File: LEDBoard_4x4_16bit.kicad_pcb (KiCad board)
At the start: 2 copper layers, 40 x 40 mm, 35 parts, among them J1 signal_in, J2 power, J6 signal_out, U1 TLC5971RGER, U2 TLC5971RGER, U3 TLC5971RGER, U4 TLC5971RGER

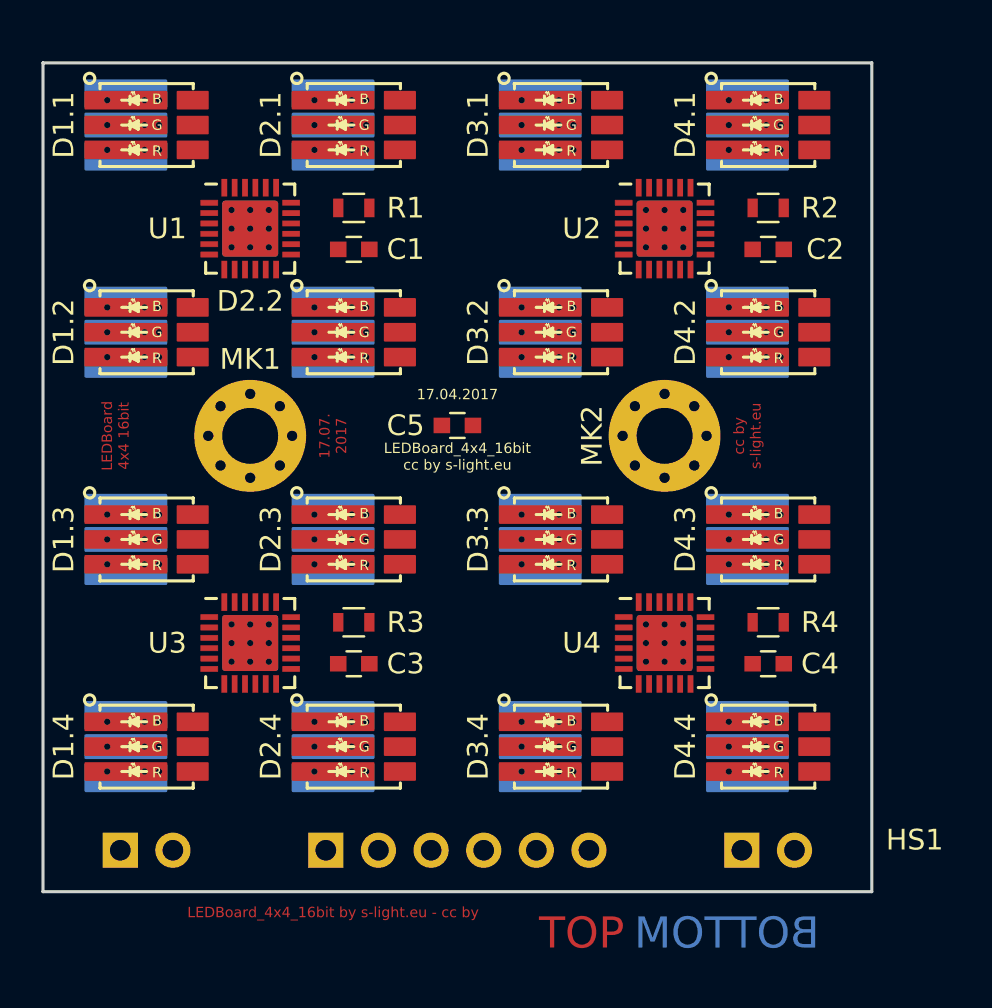
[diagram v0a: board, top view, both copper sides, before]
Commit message: pcb started routing
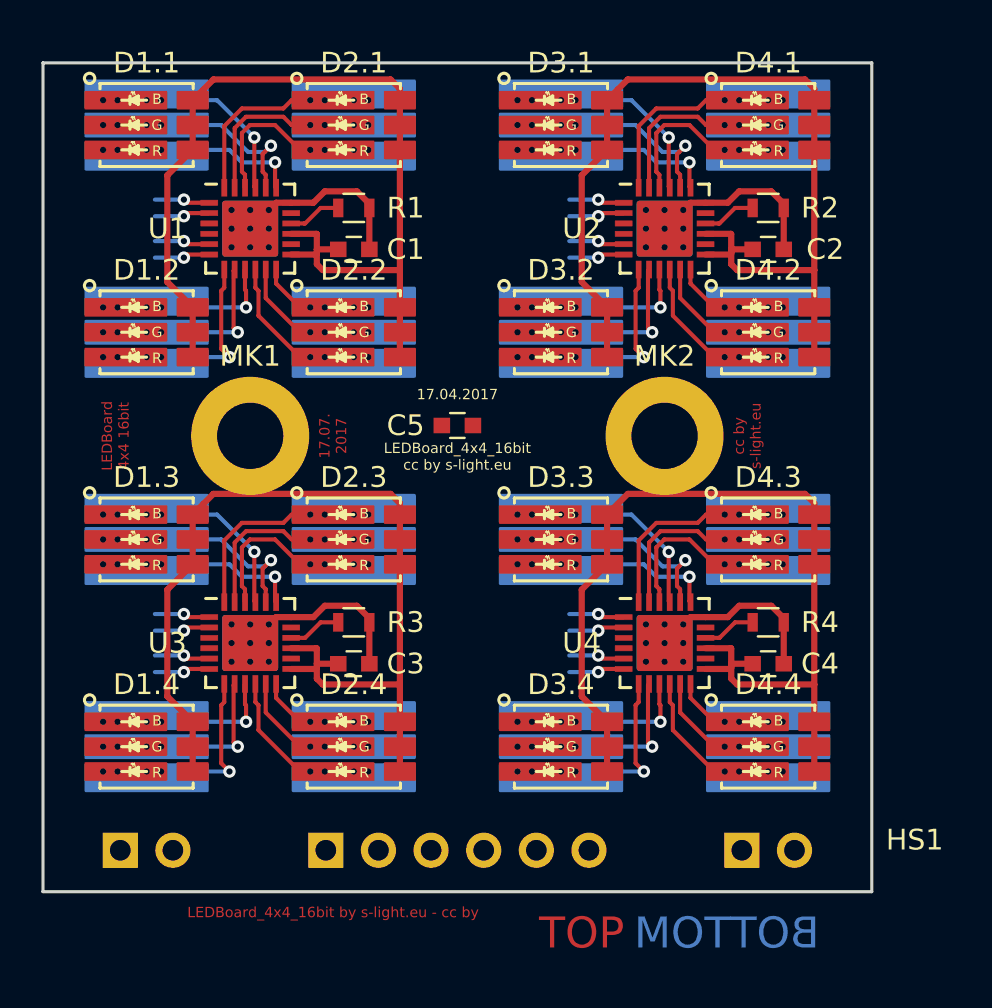
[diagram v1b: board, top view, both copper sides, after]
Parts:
- D1.1, D1.2, D1.3, D1.4, D2.1, D2.2, D2.3, D2.4, D3.1, D3.2, D3.3, D3.4, D4.1, D4.2, D4.3, D4.4: footprint nichia:LED_NSSM032AT_wViaHeatSink -> nichia:LED_NSSM032AT_wViaHeatSinkBig
- MK1, MK2: footprint Mounting_Holes:MountingHole_2.7mm_M2.5_Pad_Via -> Mounting_Holes:MountingHole_3.2mm_M3_ISO7380_Pad
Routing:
- net VCC: track 0.00 -> 184.3 mm
- net GND: track 0.00 -> 88.3 mm
- net /LED_3.1_G: track 0.00 -> 35.7 mm, vias 0 -> 4
- net /LED_4.1_B: track 0.00 -> 35.0 mm
- net /LED_3.2_R: track 0.00 -> 33.8 mm, vias 0 -> 4
- net /LED_3.1_B: track 0.00 -> 33.6 mm, vias 0 -> 4
- net /LED_4.1_G: track 0.00 -> 32.1 mm
- net /LED_4.1_R: track 0.00 -> 31.0 mm
- net /LED_3.1_R: track 0.00 -> 30.8 mm, vias 0 -> 4
- net /LED_3.2_G: track 0.00 -> 30.1 mm, vias 0 -> 4
- net /LED_4.2_R: track 0.00 -> 28.1 mm
- net /LED_3.2_B: track 0.00 -> 26.6 mm, vias 0 -> 4
- net /LED_4.2_G: track 0.00 -> 22.4 mm
- net /LED_4.2_B: track 0.00 -> 16.8 mm
- net Net-(U2-Pad6): track 0.00 -> 10.7 mm, vias 0 -> 4
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
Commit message: pcb routing almost finished
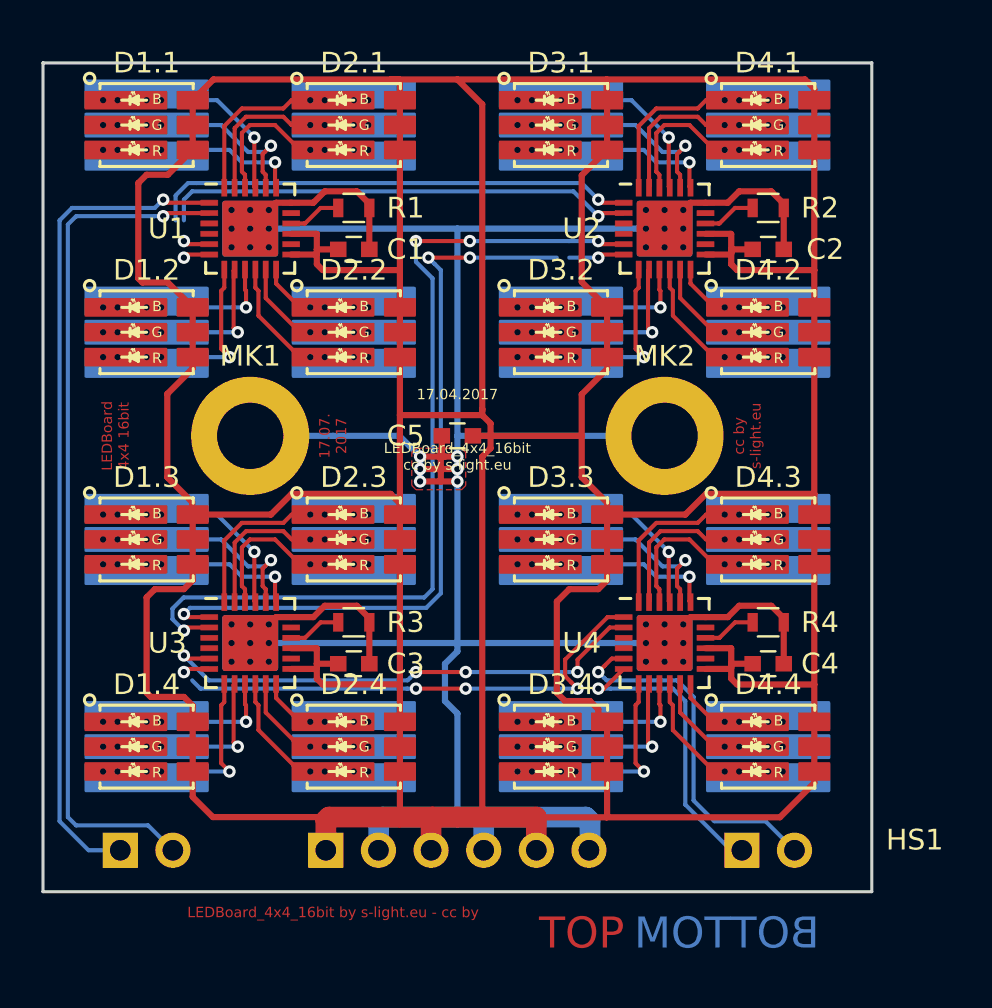
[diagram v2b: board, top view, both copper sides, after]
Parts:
- moved C5 0.50 mm to (70.0, 68.0)
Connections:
- U4 pad 6: Net-(U4-Pad6) -> /data_out
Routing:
- net VCC: track 184.3 -> 325.1 mm
- net GND: track 88.3 -> 199.4 mm, vias 0 -> 6
- net /clock_in: track 0.00 -> 41.4 mm, vias 0 -> 1
- net /data_in: track 0.00 -> 40.4 mm, vias 0 -> 1
- net /data_1-2: track 0.00 -> 36.7 mm, vias 0 -> 3
- net /clock_1-2: track 10.7 -> 42.7 mm
- net /LED_3.1_G: track 35.7 -> 8.92 mm, vias 4 -> 1
- net /LED_4.1_B: track 35.0 -> 8.74 mm
- net /LED_3.2_R: track 33.8 -> 8.45 mm, vias 4 -> 1
- net /LED_3.1_B: track 33.6 -> 8.39 mm, vias 4 -> 1
- net /clock_2-3: track 0.00 -> 24.6 mm, vias 0 -> 4
- net /data_2-3: track 0.00 -> 24.5 mm, vias 0 -> 3
- net /LED_4.1_G: track 32.1 -> 8.02 mm
- net /LED_4.1_R: track 31.0 -> 7.76 mm
- net /LED_3.1_R: track 30.8 -> 7.69 mm, vias 4 -> 1
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- added copper zone on F.Cu, net GND
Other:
- net class signal added: clearance 0.15, trace_width 0.2, via_dia 0.6, via_drill 0.3
